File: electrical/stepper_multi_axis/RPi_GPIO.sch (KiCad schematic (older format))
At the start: 7 parts, among them J35 MICROMOD-2222-C, J36 Conn_01x02_Male, J37 Conn_01x02_Male

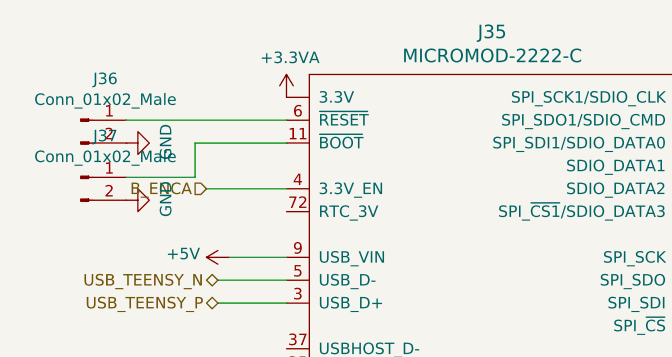
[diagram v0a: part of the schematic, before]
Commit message: bunches of changes
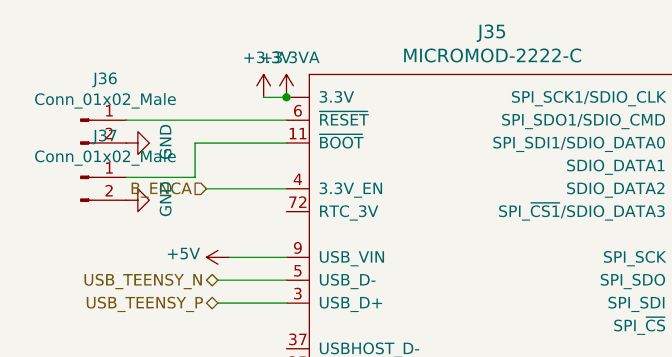
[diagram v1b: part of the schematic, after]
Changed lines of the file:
@@
 Wire Wire Line
 	4800 4200 4950 4200
+$Comp
+L power:+3.3V #PWR0101
+U 1 1 616D7C7A
+P 4850 1800
+F 0 "#PWR0101" H 4850 1650 50  0001 C CNN
+F 1 "+3.3V" H 4865 1973 50  0000 C CNN
+F 2 "" H 4850 1800 50  0001 C CNN
+F 3 "" H 4850 1800 50  0001 C CNN
+	1    4850 1800
+	1    0    0    -1
+$EndComp
+Wire Wire Line
+	4850 1800 4950 1800
+Connection ~ 4950 1800
 $EndSCHEMATC
